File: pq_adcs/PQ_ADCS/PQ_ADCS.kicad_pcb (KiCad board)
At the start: 6 copper layers, 40 x 40 mm, 55 parts, among them J1 CES-110-02-L-S, J10 Pico-Clasp_01x09, J11 Pico-Clasp_01x15, J12 CES-102-02-L-S, J2 CES-110-02-L-S, J3 CES-110-02-L-S, J4 CES-110-02-L-S, J5 Pico-Clasp_01x03, J6 Pico-Clasp_01x10, J7 Pico-Clasp_01x10, J8 Pico-Clasp_01x10, J9 Pico-Clasp_01x10, U1 LPV542, U2 LPV542, U3 LPV542, U4 IIM-42652, U5 BD2606MVV, U6 TMUX1108RSVR, U7 TCN75AVOA713

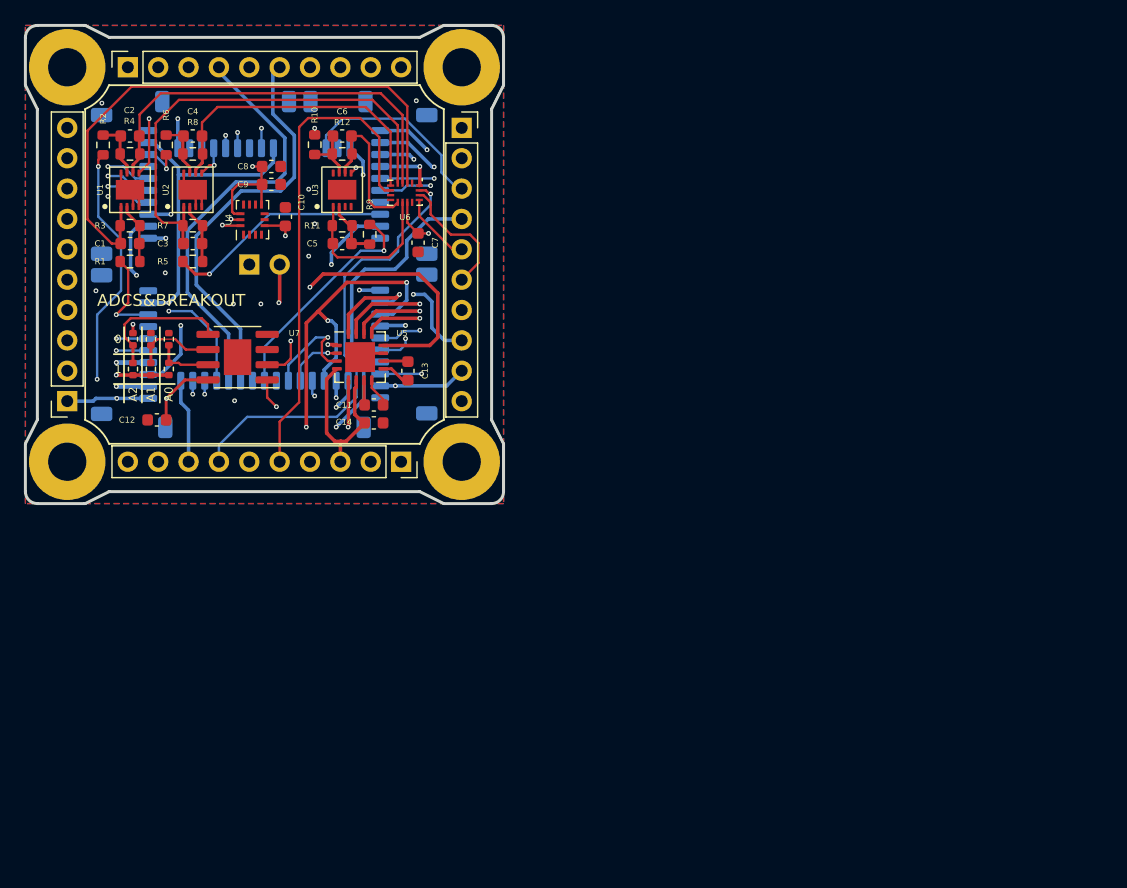
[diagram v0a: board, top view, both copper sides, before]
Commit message: document formating
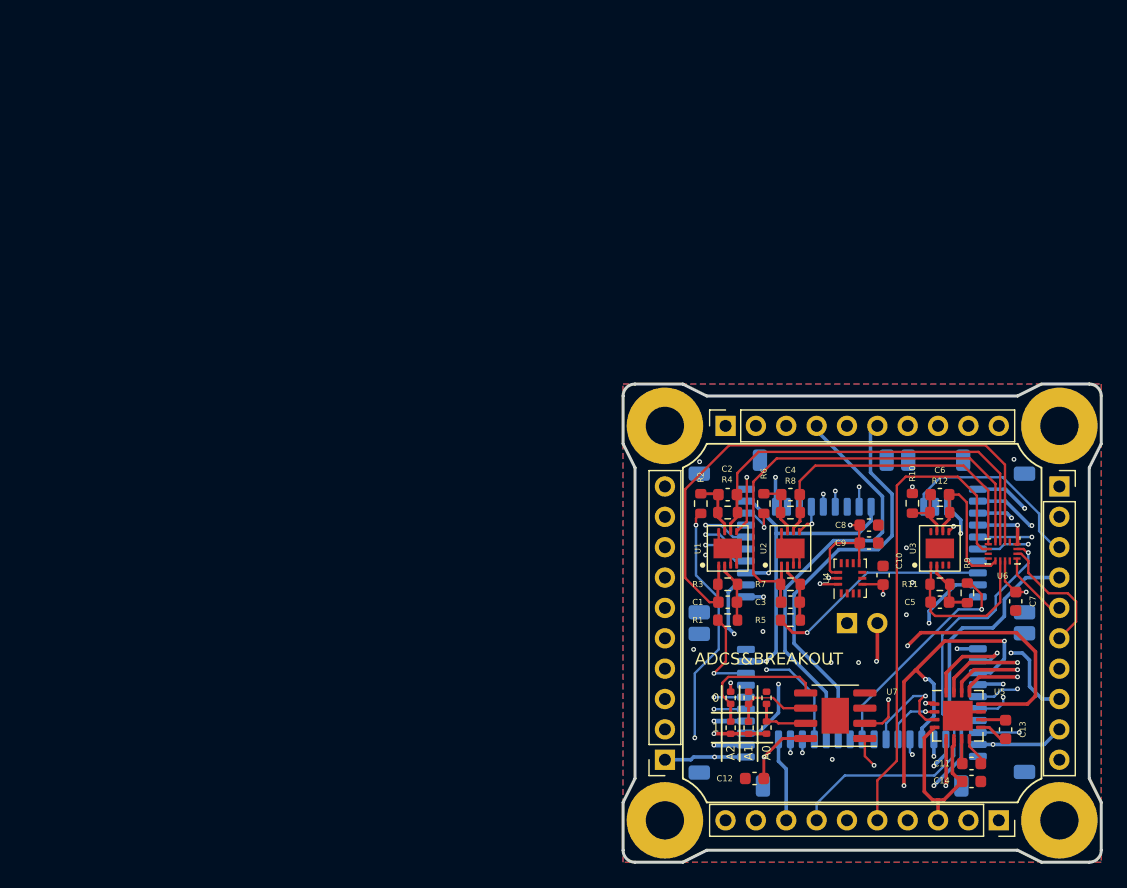
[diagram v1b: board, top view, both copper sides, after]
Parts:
- moved J7 58.3 mm to (161.7, 101.7)
- moved J8 58.3 mm to (161.7, 88.3)
- moved R9 58.3 mm to (158.8, 92.5)
- moved J10 58.3 mm to (146.8, 83.2)
- moved J5 58.3 mm to (156.2, 83.2)
- moved C1 58.3 mm to (138.8, 93.2)
- moved C10 58.3 mm to (151.8, 91.0)
- moved C11 58.3 mm to (159.2, 108.2)
- moved C12 58.3 mm to (141.0, 108.0)
- moved C13 58.3 mm to (162.0, 103.9)
- moved C14 58.3 mm to (159.2, 106.8)
- moved C2 58.3 mm to (138.8, 84.2)
- moved C3 58.3 mm to (144.0, 93.2)
- moved C4 58.3 mm to (144.0, 84.2)
- moved C5 58.3 mm to (156.5, 93.2)
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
